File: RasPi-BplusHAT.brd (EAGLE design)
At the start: 65 x 56 mm, 7 parts, among them K1 PIN20X2, U1 EEPROM24

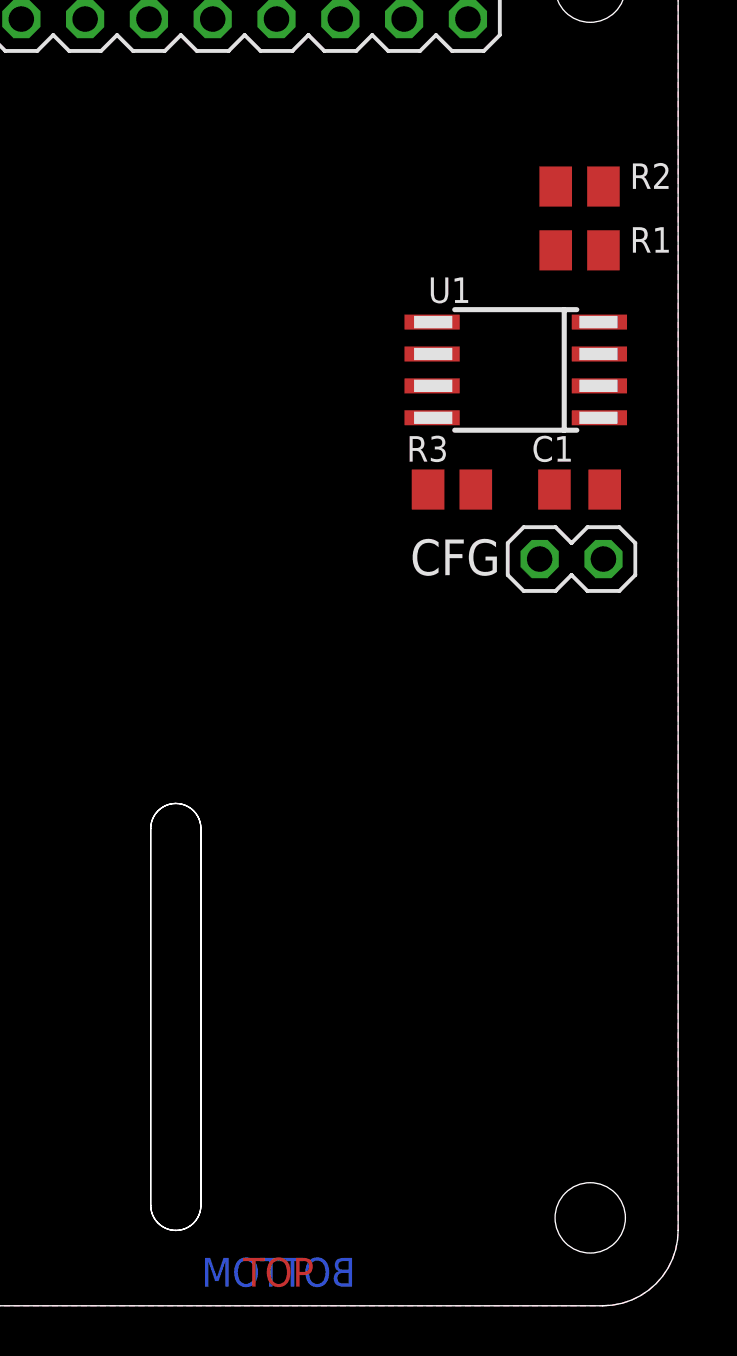
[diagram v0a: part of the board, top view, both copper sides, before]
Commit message: delete cruft
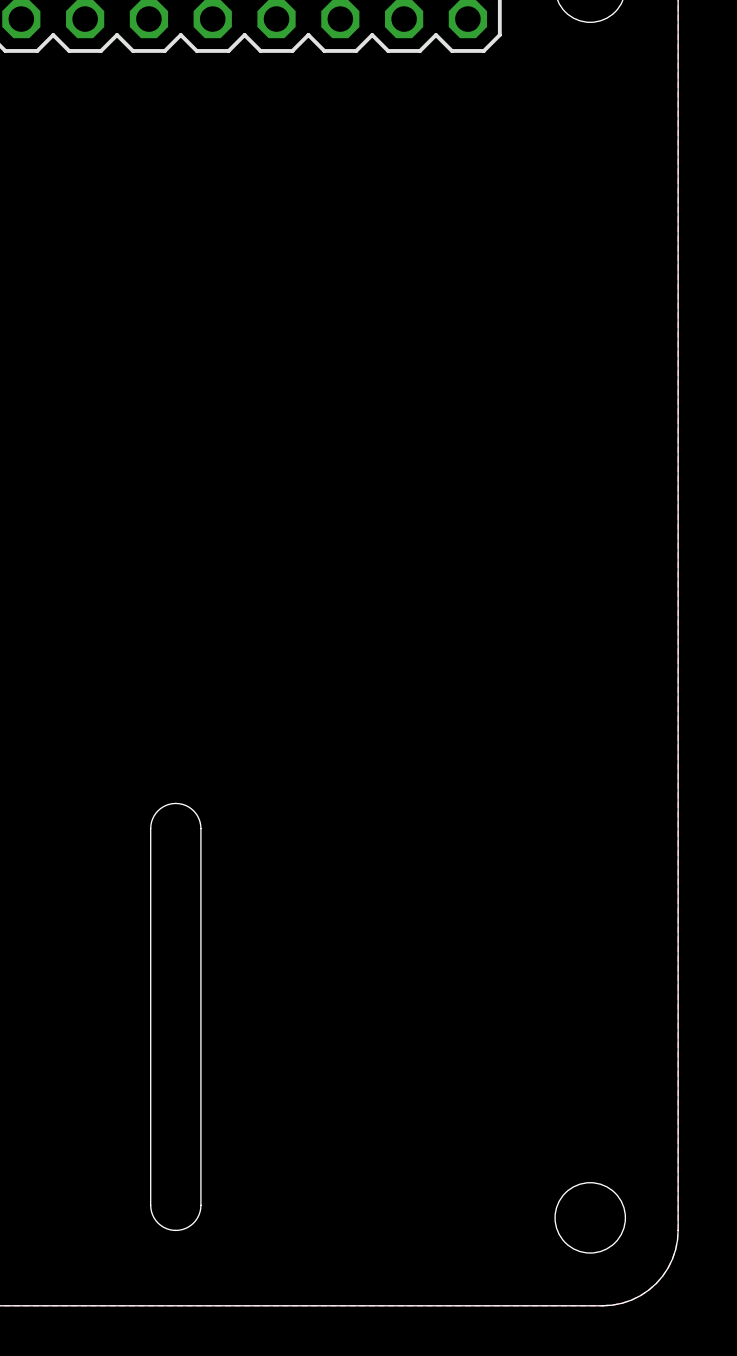
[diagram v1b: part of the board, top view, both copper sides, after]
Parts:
- removed C1: 100nF, resistor:C0805K
- removed CFG: (no value), FLYFISH:PIN_W_2
- removed R1, R2: 3k9, resistor:M0805
- removed R3: 1k, resistor:M0805
- removed U1: EEPROM24, FLYFISH:SOIC8
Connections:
- removed net N$1: K1.28, R1.1, U1.6
- removed net N$2: K1.27, R2.1, U1.5
- removed net N$3: CFG.1, R3.1, U1.7
- net +3V3: no longer C1.1, R1.2, R2.2, R3.2, U1.8
- net GND: no longer C1.2, CFG.2, U1.1, U1.2, U1.3, U1.4
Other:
- board text removed: "BOTTOM"
- board text removed: "TOP"
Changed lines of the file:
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@@
 <hole x="61.5" y="52.5" drill="2.8"/>
 <hole x="61.5" y="3.5" drill="2.8"/>
-<text x="49.09" y="1.335" size="1.143" layer="1" font="vector" ratio="23" rot="SR0" align="center">TOP</text>
-<text x="49.09" y="1.335" size="1.143" layer="16" font="vector" ratio="23" rot="SMR0" align="center">BOTTOM</text>
 <circle x="3.5" y="52.5" radius="1.55" width="3.1" layer="41"/>
 <circle x="61.5" y="52.5" radius="1.55" width="3.1" layer="41"/>
@@
 <wire x1="45" y1="20" x2="46" y2="19" width="0" layer="46" curve="-90"/>
 <wire x1="46" y1="19" x2="46" y2="4" width="0" layer="46"/>
-<wire x1="44" y1="19" x2="44" y2="4" width="0" layer="20"/>
-<wire x1="46" y1="19" x2="46" y2="4" width="0" layer="20"/>
-<wire x1="45" y1="20" x2="46" y2="19" width="0" layer="20" curve="-90"/>
-<wire x1="45" y1="20" x2="44" y2="19" width="0" layer="20" curve="90"/>
-<wire x1="46" y1="4" x2="45" y2="3" width="0" layer="20" curve="-90"/>
-<wire x1="44" y1="4" x2="45" y2="3" width="0" layer="20" curve="90"/>
 </plain>
 <attributes>
@@
 <attribute name="VALUE" x="45.2" y="48.309" size="1.27" layer="27" ratio="10"/>
 </element>
-<element name="U1" library="FLYFISH" package="SOIC8" value="EEPROM24" x="58.535" y="37.26" smashed="yes" rot="R90">
-<attribute name="NAME" x="55.0425" y="39.927" size="1.016" layer="25" ratio="10"/>
-<attribute name="VALUE" x="57.265" y="39.9905" size="0.8128" layer="27"/>
-</element>
-<element name="R1" library="resistor" package="M0805" value="3k9" x="61.075" y="42.0225" smashed="yes">
-<attribute name="TOLERANCE" value="5%" x="61.075" y="42.0225" size="1.778" layer="27" display="off"/>
-<attribute name="NAME" x="63.07525" y="41.92725" size="1.016" layer="25" ratio="10"/>
-<attribute name="VALUE" x="62.9165" y="41.0065" size="0.8128" layer="27"/>
-</element>
-<element name="C1" library="resistor" package="C0805K" value="100nF" x="61.075" y="32.4975" smashed="yes">
-<attribute name="DIELECTRIC" value="X7R" x="61.075" y="32.4975" size="1.778" layer="27" display="off"/>
-<attribute name="NAME" x="59.17" y="33.60875" size="1.016" layer="25" ratio="10"/>
-<attribute name="VALUE" x="61.0275" y="33.7675" size="0.8128" layer="27"/>
-</element>
-<element name="R2" library="resistor" package="M0805" value="3k9" x="61.075" y="44.5625" smashed="yes">
-<attribute name="TOLERANCE" value="5%" x="61.075" y="44.5625" size="1.778" layer="27" display="off"/>
-<attribute name="NAME" x="63.07525" y="44.46725" size="1.016" layer="25" ratio="10"/>
-<attribute name="VALUE" x="62.9165" y="43.5465" size="0.8128" layer="27"/>
-</element>
-<element name="R3" library="resistor" package="M0805" value="1k" x="55.995" y="32.4975" smashed="yes">
-<attribute name="TOLERANCE" value="5%" x="55.995" y="32.4975" size="1.778" layer="27" display="off"/>
-<attribute name="NAME" x="54.18525" y="33.60875" size="1.016" layer="25" ratio="10"/>
-<attribute name="VALUE" x="56.40775" y="33.7675" size="0.8128" layer="27"/>
-</element>
-<element name="CFG" library="FLYFISH" package="PIN_W_2" value="" x="59.485" y="29.73" smashed="yes" rot="R90">
-<attribute name="NAME" x="54.3313" y="29.08755" size="1.4224" layer="25" ratio="15"/>
-<attribute name="VALUE" x="65.2" y="28.46" size="1.27" layer="27" rot="R90"/>
-</element>
 </elements>
 <signals>
@@
 </signal>
 <signal name="GND">
-<contactref element="U1" pad="4"/>
-<contactref element="U1" pad="3"/>
-<contactref element="U1" pad="1"/>
-<contactref element="U1" pad="2"/>
-<contactref element="CFG" pad="2"/>
-<contactref element="C1" pad="2"/>
 <contactref element="K1" pad="9"/>
 <contactref element="K1" pad="25"/>
@@
 <vertex x="0" y="18.5"/>
 </polygon>
+<wire x1="49.01" y1="53.77" x2="56.63" y2="51.23" width="0" layer="19" extent="1-1"/>
+<wire x1="43.93" y1="53.77" x2="49.01" y2="53.77" width="0" layer="19" extent="1-1"/>
+<wire x1="38.85" y1="51.23" x2="43.93" y2="53.77" width="0" layer="19" extent="1-1"/>
+<wire x1="31.23" y1="53.77" x2="38.85" y2="51.23" width="0" layer="19" extent="1-1"/>
+<wire x1="23.61" y1="53.77" x2="31.23" y2="53.77" width="0" layer="19" extent="1-1"/>
+<wire x1="18.53" y1="51.23" x2="23.61" y2="53.77" width="0" layer="19" extent="1-1"/>
+<wire x1="13.45" y1="53.77" x2="18.53" y2="51.23" width="0" layer="19" extent="1-1"/>
 </signal>
 <signal name="+3V3">
-<contactref element="U1" pad="8"/>
-<contactref element="R3" pad="2"/>
-<contactref element="C1" pad="1"/>
-<contactref element="R2" pad="2"/>
-<contactref element="R1" pad="2"/>
 <contactref element="K1" pad="1"/>
 <contactref element="K1" pad="17"/>
-<wire x1="62.025" y1="42.0225" x2="62.025" y2="44.5625" width="0" layer="19" extent="1-1"/>
-<wire x1="55.205" y1="35.355" x2="62.025" y2="42.0225" width="0" layer="19" extent="1-1"/>
-<wire x1="56.945" y1="32.4975" x2="55.205" y2="35.355" width="0" layer="19" extent="1-1"/>
-<wire x1="60.075" y1="32.4975" x2="56.945" y2="32.4975" width="0" layer="19" extent="1-1"/>
-<wire x1="28.69" y1="51.23" x2="55.205" y2="35.355" width="0" layer="19" extent="1-1"/>
 <wire x1="8.37" y1="51.23" x2="28.69" y2="51.23" width="0" layer="19" extent="1-1"/>
 </signal>
-<signal name="N$1">
-<contactref element="U1" pad="6"/>
-<contactref element="R1" pad="1"/>
-<contactref element="K1" pad="28"/>
-<wire x1="55.205" y1="37.895" x2="60.125" y2="42.0225" width="0" layer="19" extent="1-1"/>
-<wire x1="41.39" y1="53.77" x2="55.205" y2="37.895" width="0" layer="19" extent="1-1"/>
-</signal>
-<signal name="N$2">
-<contactref element="U1" pad="5"/>
-<contactref element="R2" pad="1"/>
-<contactref element="K1" pad="27"/>
-<wire x1="55.205" y1="39.165" x2="60.125" y2="44.5625" width="0" layer="19" extent="1-1"/>
-<wire x1="41.39" y1="51.23" x2="55.205" y2="39.165" width="0" layer="19" extent="1-1"/>
-</signal>
-<signal name="N$3">
-<contactref element="U1" pad="7"/>
-<contactref element="R3" pad="1"/>
-<contactref element="CFG" pad="1"/>
-<wire x1="55.045" y1="32.4975" x2="55.205" y2="36.625" width="0" layer="19" extent="1-1"/>
-<wire x1="59.485" y1="29.73" x2="55.045" y2="32.4975" width="0" layer="19" extent="1-1"/>
-</signal>
 <signal name="+5V">
